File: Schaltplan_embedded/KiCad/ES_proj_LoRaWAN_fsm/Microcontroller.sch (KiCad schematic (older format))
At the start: 15 parts, among them J1 Conn_02x05_Odd_Even, SW1 SW_Push, U1 STM32L476RGTx, Y1 Crystal

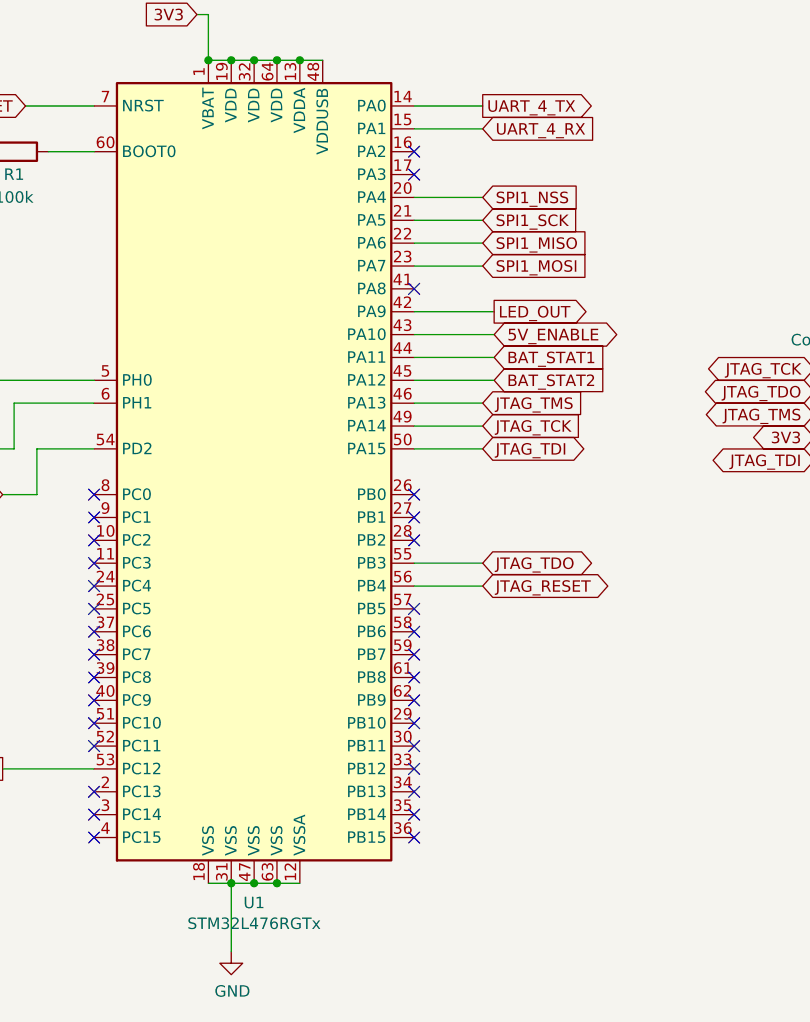
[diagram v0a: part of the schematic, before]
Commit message: schaltplan neu
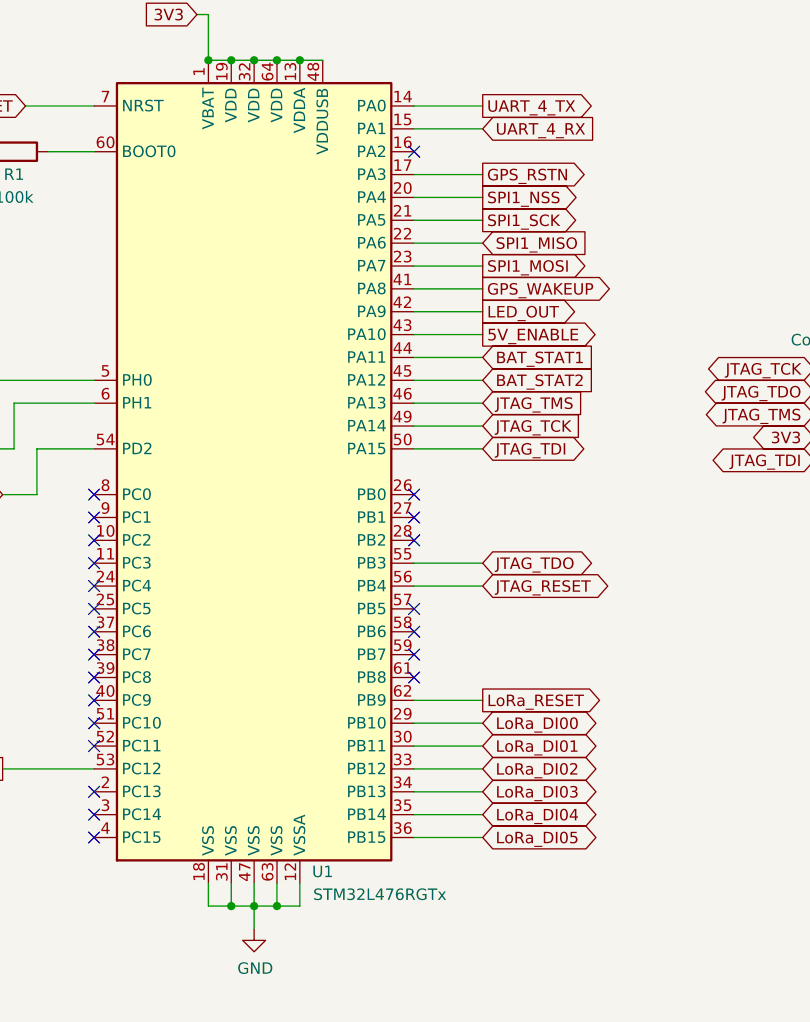
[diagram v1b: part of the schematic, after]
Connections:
- net labels added: GPS_RSTN, GPS_WAKEUP, LoRa_DI00, LoRa_DI01, LoRa_DI02, LoRa_DI03, LoRa_DI04, LoRa_DI05, LoRa_RESET
- wire segments 77 -> 91
- no-connect marks 34 -> 25
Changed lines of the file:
@@
 L power:GND #PWR0102
 U 1 1 5DC1AD63
-P 4000 6750
-F 0 "#PWR0102" H 4000 6500 50  0001 C CNN
-F 1 "GND" H 4005 6577 50  0000 C CNN
-F 2 "" H 4000 6750 50  0001 C CNN
-F 3 "" H 4000 6750 50  0001 C CNN
-	1    4000 6750
-	1    0    0    -1
-$EndComp
-Wire Wire Line
-	4000 6450 3900 6450
-Connection ~ 4000 6450
-Wire Wire Line
-	4000 6450 4000 6750
+P 4100 6650
+F 0 "#PWR0102" H 4100 6400 50  0001 C CNN
+F 1 "GND" H 4105 6477 50  0000 C CNN
+F 2 "" H 4100 6650 50  0001 C CNN
+F 3 "" H 4100 6650 50  0001 C CNN
+	1    4100 6650
+	1    0    0    -1
+$EndComp
 Text GLabel 4850 1300 0    50   Input ~ 0
 3V3
@@
 Wire Wire Line
 	6400 1300 6400 1400
-Text GLabel 5100 3450 2    50   Input ~ 0
+Text GLabel 5100 3450 2    50   Output ~ 0
 SPI1_NSS
 Wire Wire Line
 	4800 3450 5100 3450
-Text GLabel 5100 3550 2    50   Input ~ 0
+Text GLabel 5100 3550 2    50   Output ~ 0
 SPI1_SCK
 Wire Wire Line
@@
 Text GLabel 5100 3650 2    50   Input ~ 0
 SPI1_MISO
-Text GLabel 5100 3750 2    50   Input ~ 0
+Text GLabel 5100 3750 2    50   Output ~ 0
 SPI1_MOSI
-Wire Wire Line
-	4300 6450 4200 6450
-Connection ~ 4200 6450
-Wire Wire Line
-	4100 6450 4000 6450
-Wire Wire Line
-	4100 6450 4200 6450
-Connection ~ 4100 6450
-Wire Wire Line
-	4300 2850 4400 2850
-Connection ~ 4300 2850
-Wire Wire Line
-	4200 2850 4300 2850
-Connection ~ 4200 2850
-Wire Wire Line
-	4100 2850 4200 2850
-Connection ~ 4100 2850
-Wire Wire Line
-	4100 2850 4000 2850
-Wire Wire Line
-	3900 2850 4000 2850
-Connection ~ 4000 2850
-Connection ~ 3900 2850
-$Comp
-L MCU_ST_STM32L4:STM32L476RGTx U1
-U 1 1 5DC1A60F
-P 4100 4650
-F 0 "U1" H 4100 2764 50  0000 C CNN
-F 1 "STM32L476RGTx" H 4100 2673 50  0000 C CNN
-F 2 "Package_QFP:LQFP-64_10x10mm_P0.5mm" H 3500 2950 50  0001 R CNN
-F 3 "http://www.st.com/st-web-ui/static/active/en/resource/technical/document/datasheet/DM00108832.pdf" H 4100 4650 50  0001 C CNN
-	1    4100 4650
-	1    0    0    -1
-$EndComp
 Wire Wire Line
 	4800 3650 5100 3650
@@
 Wire Wire Line
 	2700 3250 2700 3350
-Text GLabel 5150 3950 2    50   Output ~ 0
+Text GLabel 5100 3950 2    50   Output ~ 0
 LED_OUT
 Wire Wire Line
-	5150 3950 4800 3950
+	5100 3950 4800 3950
 Text GLabel 8600 4350 0    50   Input ~ 0
 LED_OUT
@@
 Wire Wire Line
 	9550 4350 9850 4350
-Text GLabel 5150 4050 2    51   BiDi ~ 0
+Text GLabel 5100 4050 2    51   Output ~ 0
 5V_ENABLE
 Wire Wire Line
-	5150 4050 4800 4050
-NoConn ~ 4800 6250
-NoConn ~ 4800 6150
-NoConn ~ 4800 6050
-NoConn ~ 4800 5950
-NoConn ~ 4800 5850
-NoConn ~ 4800 5750
-NoConn ~ 4800 5650
+	5100 4050 4800 4050
 NoConn ~ 4800 5550
 NoConn ~ 4800 5450
@@
 NoConn ~ 4800 4850
 NoConn ~ 4800 4750
-NoConn ~ 4800 3850
-NoConn ~ 4800 3350
 NoConn ~ 4800 3250
 Text GLabel 3100 3050 0    50   Input ~ 0
@@
 Wire Wire Line
 	3400 3050 3100 3050
-Text GLabel 5150 4150 2    50   Input ~ 0
+Text GLabel 5100 4150 2    50   Input ~ 0
 BAT_STAT1
-Text GLabel 5150 4250 2    50   Input ~ 0
+Text GLabel 5100 4250 2    50   Input ~ 0
 BAT_STAT2
 Wire Wire Line
-	4800 4150 5150 4150
-Wire Wire Line
-	4800 4250 5150 4250
+	4800 4150 5100 4150
+Wire Wire Line
+	4800 4250 5100 4250
+Text GLabel 5100 3850 2    50   Output ~ 0
+GPS_WAKEUP
+Wire Wire Line
+	4800 3850 5100 3850
+Text GLabel 5100 3350 2    50   Output ~ 0
+GPS_RSTN
+Wire Wire Line
+	4800 3350 5100 3350
+Text GLabel 5100 5850 2    50   BiDi ~ 0
+LoRa_DI01
+Text GLabel 5100 5750 2    50   BiDi ~ 0
+LoRa_DI00
+Text GLabel 5100 5950 2    50   BiDi ~ 0
+LoRa_DI02
+Text GLabel 5100 6050 2    50   BiDi ~ 0
+LoRa_DI03
+Text GLabel 5100 6150 2    50   BiDi ~ 0
+LoRa_DI04
+Text GLabel 5100 6250 2    50   BiDi ~ 0
+LoRa_DI05
+Wire Wire Line
+	4800 5750 5100 5750
+Wire Wire Line
+	4800 5850 5100 5850
+Wire Wire Line
+	4800 5950 5100 5950
+Wire Wire Line
+	4800 6050 5100 6050
+Wire Wire Line
+	4800 6150 5100 6150
+Wire Wire Line
+	4800 6250 5100 6250
+Text GLabel 5100 5650 2    50   Output ~ 0
+LoRa_RESET
+Wire Wire Line
+	4800 5650 5100 5650
+Wire Wire Line
+	4300 2850 4400 2850
+Connection ~ 4300 2850
+Wire Wire Line
+	4200 2850 4300 2850
+Connection ~ 4200 2850
+Wire Wire Line
+	4100 2850 4200 2850
+Connection ~ 4100 2850
+Wire Wire Line
+	3900 2850 4000 2850
+Wire Wire Line
+	4100 2850 4000 2850
+Connection ~ 4000 2850
+Connection ~ 3900 2850
+$Comp
+L MCU_ST_STM32L4:STM32L476RGTx U1
+U 1 1 5DC1A60F
+P 4100 4650
+F 0 "U1" H 4400 2900 50  0000 C CNN
+F 1 "STM32L476RGTx" H 4650 2800 50  0000 C CNN
+F 2 "Package_QFP:LQFP-64_10x10mm_P0.5mm" H 3500 2950 50  0001 R CNN
+F 3 "http://www.st.com/st-web-ui/static/active/en/resource/technical/document/datasheet/DM00108832.pdf" H 4100 4650 50  0001 C CNN
+	1    4100 4650
+	1    0    0    -1
+$EndComp
+Wire Wire Line
+	3900 6450 3900 6550
+Wire Wire Line
+	3900 6550 4000 6550
+Wire Wire Line
+	4300 6550 4300 6450
+Wire Wire Line
+	4000 6450 4000 6550
+Connection ~ 4000 6550
+Wire Wire Line
+	4000 6550 4100 6550
+Wire Wire Line
+	4100 6450 4100 6550
+Connection ~ 4100 6550
+Wire Wire Line
+	4100 6550 4200 6550
+Wire Wire Line
+	4200 6450 4200 6550
+Connection ~ 4200 6550
+Wire Wire Line
+	4200 6550 4300 6550
+Wire Wire Line
+	4100 6550 4100 6650
 $EndSCHEMATC

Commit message: Pin_änderung_KeinPush
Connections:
- net labels added: USART_2_TX, USART_3_RX
- no-connect marks 25 -> 19
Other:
- note added: "Conexion para comunicacion seral con PC, conectar a Conn de 2 pines\n"
- note added: "Cuadrar estos\n"
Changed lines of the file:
@@
 Wire Wire Line
 	6400 1300 6400 1400
-Text GLabel 5100 3450 2    50   Output ~ 0
+Text GLabel 5100 5350 2    50   Output ~ 0
 SPI1_NSS
-Wire Wire Line
-	4800 3450 5100 3450
 Text GLabel 5100 3550 2    50   Output ~ 0
 SPI1_SCK
@@
 Wire Wire Line
 	2700 3250 2700 3350
-Text GLabel 5100 3950 2    50   Output ~ 0
+Text GLabel 3000 5650 0    50   Output ~ 0
 LED_OUT
-Wire Wire Line
-	5100 3950 4800 3950
 Text GLabel 8600 4350 0    50   Input ~ 0
 LED_OUT
@@
 Wire Wire Line
 	9550 4350 9850 4350
-Text GLabel 5100 4050 2    51   Output ~ 0
+Text GLabel 5100 5600 2    51   Output ~ 0
 5V_ENABLE
-Wire Wire Line
-	5100 4050 4800 4050
 NoConn ~ 4800 5550
 NoConn ~ 4800 5450
-NoConn ~ 4800 5350
 NoConn ~ 4800 5250
 NoConn ~ 3400 6250
@@
 NoConn ~ 3400 5850
 NoConn ~ 3400 5750
-NoConn ~ 3400 5650
 NoConn ~ 3400 5550
-NoConn ~ 3400 5450
 NoConn ~ 3400 5350
-NoConn ~ 3400 5250
-NoConn ~ 3400 5150
 NoConn ~ 3400 5050
 NoConn ~ 3400 4950
@@
 NoConn ~ 4800 4850
 NoConn ~ 4800 4750
-NoConn ~ 4800 3250
 Text GLabel 3100 3050 0    50   Input ~ 0
 JTAG_RESET
@@
 Wire Wire Line
 	4800 4250 5100 4250
-Text GLabel 5100 3850 2    50   Output ~ 0
+Text GLabel 5100 5700 2    50   Output ~ 0
 GPS_WAKEUP
-Wire Wire Line
-	4800 3850 5100 3850
 Text GLabel 5100 3350 2    50   Output ~ 0
 GPS_RSTN
 Wire Wire Line
 	4800 3350 5100 3350
-Text GLabel 5100 5850 2    50   BiDi ~ 0
+Text GLabel 5100 3950 2    50   BiDi ~ 0
 LoRa_DI01
-Text GLabel 5100 5750 2    50   BiDi ~ 0
+Text GLabel 5100 4050 2    50   BiDi ~ 0
 LoRa_DI00
-Text GLabel 5100 5950 2    50   BiDi ~ 0
+Text GLabel 5100 3850 2    50   BiDi ~ 0
 LoRa_DI02
 Text GLabel 5100 6050 2    50   BiDi ~ 0
@@
 LoRa_DI05
 Wire Wire Line
-	4800 5750 5100 5750
-Wire Wire Line
-	4800 5850 5100 5850
-Wire Wire Line
-	4800 5950 5100 5950
-Wire Wire Line
 	4800 6050 5100 6050
 Wire Wire Line
@@
 Wire Wire Line
 	4800 6250 5100 6250
-Text GLabel 5100 5650 2    50   Output ~ 0
+Text GLabel 3000 5450 0    50   Output ~ 0
 LoRa_RESET
-Wire Wire Line
-	4800 5650 5100 5650
 Wire Wire Line
 	4300 2850 4400 2850
@@
 Wire Wire Line
 	4100 6550 4100 6650
+Wire Wire Line
+	3400 5650 3000 5650
+Wire Wire Line
+	3000 5450 3400 5450
+Wire Wire Line
+	5100 3850 4800 3850
+Wire Wire Line
+	5100 3950 4800 3950
+Wire Wire Line
+	5100 4050 4800 4050
+Text Notes 5800 5700 0    50   ~ 0
+Cuadrar estos\n
+Text GLabel 3000 5150 0    50   Output ~ 0
+USART_2_TX
+Text Notes -300 5200 0    50   ~ 0
+Conexion para comunicacion seral con PC, conectar a Conn de 2 pines\n
+Wire Wire Line
+	3000 5150 3400 5150
+Text GLabel 3000 5250 0    50   Input ~ 0
+USART_3_RX
+Wire Wire Line
+	3000 5250 3400 5250
+Wire Wire Line
+	5100 5350 4800 5350
 $EndSCHEMATC
